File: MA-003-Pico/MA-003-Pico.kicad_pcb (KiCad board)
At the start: 2 copper layers, 49.5 x 80 mm, 5 parts, among them M1 rs485_ttl_module, M2 rs485_ttl_module, M3 rs485_ttl_module, M4 rs485_ttl_module

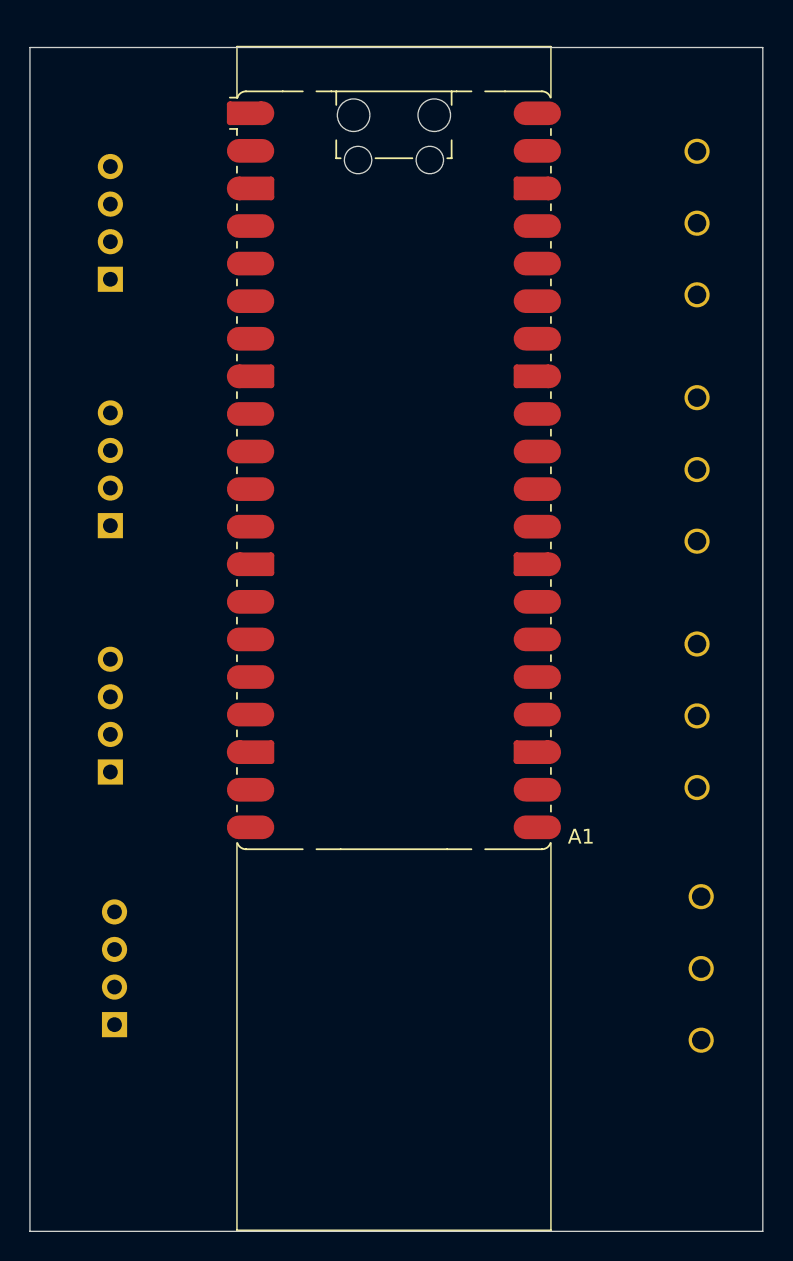
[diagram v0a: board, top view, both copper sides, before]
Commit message: Some more work
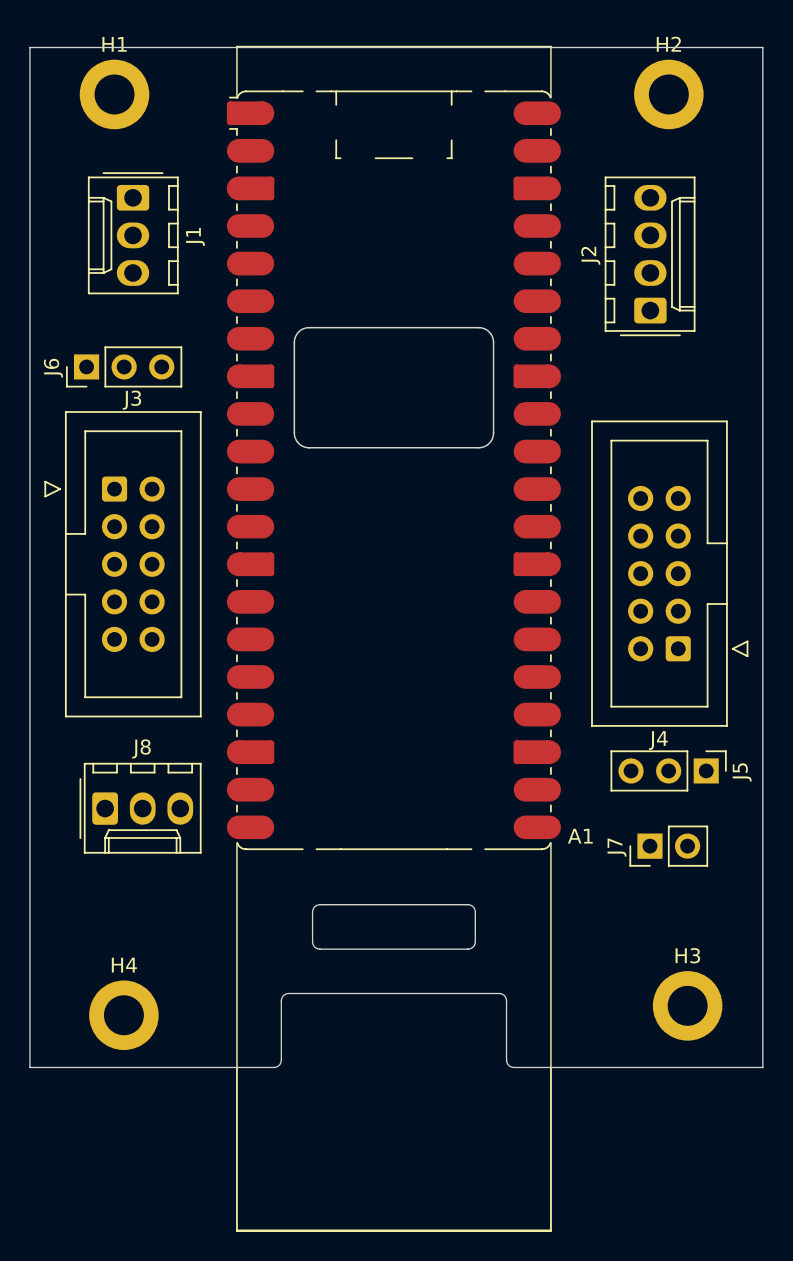
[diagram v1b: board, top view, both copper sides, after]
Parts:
- removed M1, M2, M3, M4: rs485_ttl_module, RS485ToTTL:rs485_ttl_module
- added H1: MountingHole_Pad, MountingHole:MountingHole_2.7mm_M2.5_DIN965_Pad, F.Cu at (138.4, 61.6)
- added H2: MountingHole_Pad, MountingHole:MountingHole_2.7mm_M2.5_DIN965_Pad, F.Cu at (175.9, 61.6)
- added H3: MountingHole_Pad, MountingHole:MountingHole_2.7mm_M2.5_DIN965_Pad, F.Cu at (177.2, 123.2)
- added H4: MountingHole_Pad, MountingHole:MountingHole_2.7mm_M2.5_DIN965_Pad, F.Cu at (139.1, 123.8)
- added J1: Power, Connector_Molex:Molex_KK-254_AE-6410-03A_1x03_P2.54mm_Vertical, F.Cu at (139.7, 68.6)
- added J2: I2C, Connector_Molex:Molex_KK-254_AE-6410-04A_1x04_P2.54mm_Vertical, F.Cu at (174.6, 76.2)
- added J3: Interface_A, Connector_IDC:IDC-Header_2x05_P2.54mm_Vertical, F.Cu at (138.4, 88.3)
- added J4: Interface_B, Connector_IDC:IDC-Header_2x05_P2.54mm_Vertical, F.Cu at (176.5, 99.1)
- added J5: Power_IB, Connector_PinHeader_2.54mm:PinHeader_1x03_P2.54mm_Vertical, F.Cu at (178.4, 107.3)
- added J6: Power_IA, Connector_PinHeader_2.54mm:PinHeader_1x03_P2.54mm_Vertical, F.Cu at (136.5, 80.0)
- added J7: Pico_On/Off, Connector_PinHeader_2.54mm:PinHeader_1x02_P2.54mm_Vertical, F.Cu at (174.6, 112.4)
- added J8: WS2812, Connector_Molex:Molex_KK-254_AE-6410-03A_1x03_P2.54mm_Vertical, F.Cu at (137.8, 109.9)
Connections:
- A1 pad 1: unconnected-(A1-GPIO0-Pad1) -> /GPIO_1
- A1 pad 10: unconnected-(A1-GPIO7-Pad10) -> /GPIO_8
- A1 pad 11: unconnected-(A1-GPIO8-Pad11) -> /GPIO_9
- A1 pad 12: unconnected-(A1-GPIO9-Pad12) -> /GPIO_10
- A1 pad 13: Net-(A1-GND-Pad13) -> /GND
- A1 pad 14: unconnected-(A1-GPIO10-Pad14) -> /GPIO_11
- A1 pad 15: unconnected-(A1-GPIO11-Pad15) -> /GPIO_12
- A1 pad 16: unconnected-(A1-GPIO12-Pad16) -> /GPIO_13
- A1 pad 17: unconnected-(A1-GPIO13-Pad17) -> /GPIO_14
- A1 pad 18: Net-(A1-GND-Pad13) -> /GND
- A1 pad 19: unconnected-(A1-GPIO14-Pad19) -> /GPIO_15
- A1 pad 2: unconnected-(A1-GPIO1-Pad2) -> /GPIO_2
- A1 pad 20: unconnected-(A1-GPIO15-Pad20) -> /GPIO_16
- A1 pad 23: Net-(A1-GND-Pad13) -> /GND
- A1 pad 28: Net-(A1-GND-Pad13) -> /GND
- A1 pad 3: Net-(A1-GND-Pad13) -> /GND
- A1 pad 30: unconnected-(A1-RUN-Pad30) -> Net-(A1-RUN)
- A1 pad 31: unconnected-(A1-GPIO26_ADC0-Pad31) -> /I2C_SDA
- A1 pad 32: unconnected-(A1-GPIO27_ADC1-Pad32) -> /I2C_SCL
- A1 pad 33: unconnected-(A1-AGND-Pad33) -> /GND
- A1 pad 34: unconnected-(A1-GPIO28_ADC2-Pad34) -> Net-(A1-GPIO28_ADC2)
- A1 pad 38: Net-(A1-GND-Pad13) -> /GND
- A1 pad 39: unconnected-(A1-VSYS-Pad39) -> /5V
- A1 pad 4: unconnected-(A1-GPIO2-Pad4) -> /GPIO_3
- A1 pad 5: unconnected-(A1-GPIO3-Pad5) -> /GPIO_4
- A1 pad 6: unconnected-(A1-GPIO4-Pad6) -> /GPIO_5
- A1 pad 7: unconnected-(A1-GPIO5-Pad7) -> /GPIO_6
- A1 pad 8: Net-(A1-GND-Pad13) -> /GND
- A1 pad 9: unconnected-(A1-GPIO6-Pad9) -> /GPIO_7
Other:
- board size 49.5 x 80 mm -> 49.5 x 68.9 mm

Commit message: Finishing the dmx ethernet pico
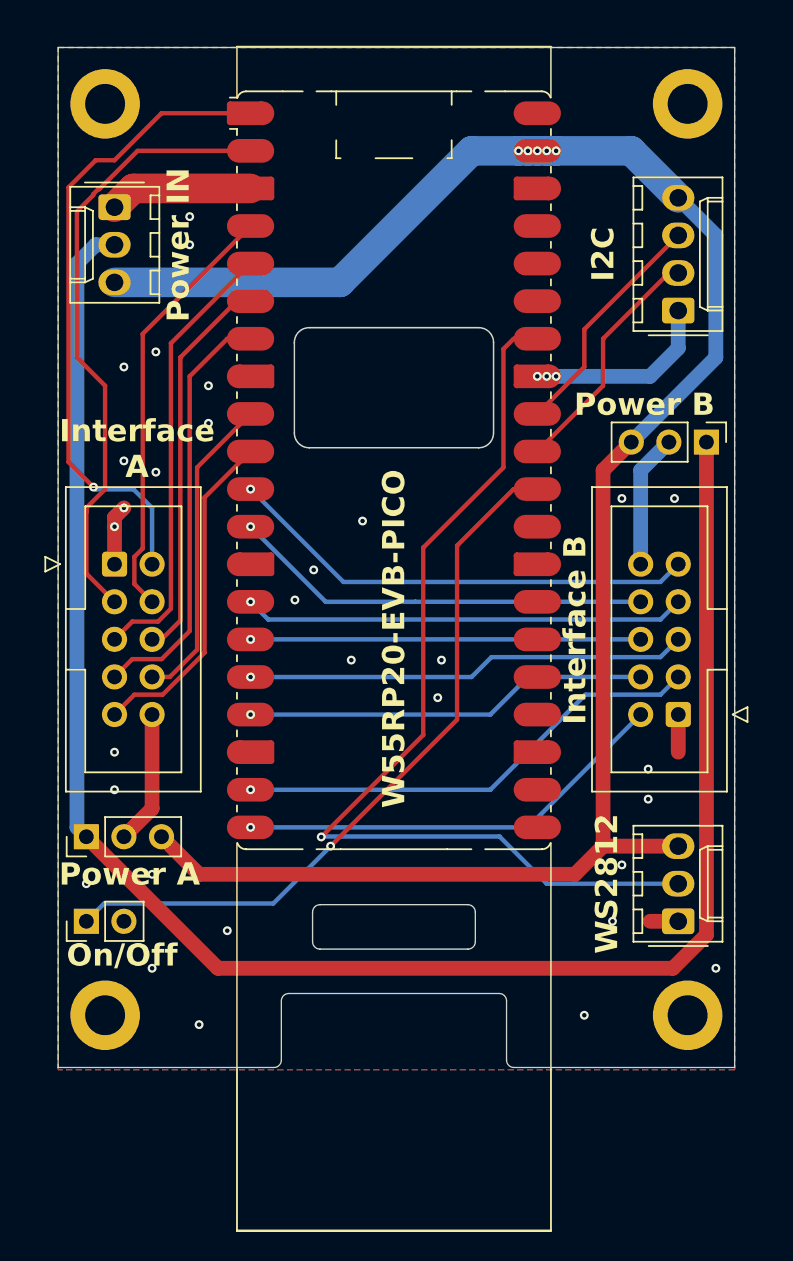
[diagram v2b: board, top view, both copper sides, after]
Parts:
- J1: value Power -> Power IN
- J3: value Interface_A -> Interface A
- moved J8 39.5 mm to (176.5, 117.5), turned to 90 degrees
- moved J7 38.4 mm to (136.5, 117.5)
- moved J6 31.8 mm to (136.5, 111.8)
- moved J5 22.2 mm to (178.4, 85.1)
- moved J3 5.08 mm to (138.4, 93.3)
- moved J4 4.44 mm to (176.5, 103.5)
- moved J2 1.88 mm to (176.5, 76.2)
- moved H2 1.42 mm to (177.2, 62.2)
- moved J1 1.40 mm to (138.4, 69.2)
- moved H4 1.27 mm to (137.8, 123.8)
- moved H1 0.90 mm to (137.8, 62.2)
- moved H3 0.64 mm to (177.2, 123.8)
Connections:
- J4 pad 2: /GPIO_9 -> /GPIO_16
- J4 pad 3: /GPIO_10 -> /GPIO_15
- J4 pad 4: /GPIO_11 -> /GPIO_14
- J4 pad 5: /GPIO_12 -> /GPIO_13
- J4 pad 6: /GPIO_13 -> /GPIO_12
- J4 pad 7: /GPIO_14 -> /GPIO_11
- J4 pad 8: /GPIO_15 -> /GPIO_10
- J4 pad 9: /GPIO_16 -> /GPIO_9
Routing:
- net /5V: track 0.00 -> 127.9 mm, vias 0 -> 5
- net /3V3: track 0.00 -> 121.9 mm
- net Net-(A1-GPIO28_ADC2): track 0.00 -> 66.1 mm, vias 0 -> 1
- net Net-(A1-RUN): track 0.00 -> 49.5 mm, vias 0 -> 1
- net /GPIO_1: track 0.00 -> 43.7 mm, vias 0 -> 1
- net /GPIO_2: track 0.00 -> 42.0 mm
- net /GPIO_15: track 0.00 -> 32.1 mm, vias 0 -> 1
- net /GPIO_9: track 0.00 -> 32.0 mm, vias 0 -> 1
- net /GND: track 0.00 -> 31.1 mm, vias 0 -> 34
- net /GPIO_4: track 0.00 -> 30.2 mm
- net /GPIO_13: track 0.00 -> 30.0 mm, vias 0 -> 1
- net /GPIO_11: track 0.00 -> 29.9 mm, vias 0 -> 1
- net /GPIO_16: track 0.00 -> 29.5 mm, vias 0 -> 1
- net /GPIO_3: track 0.00 -> 29.1 mm
- net /GPIO_6: track 0.00 -> 28.7 mm
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- added copper zone on B.Cu, net /GND
- added copper zone on F.Cu, net /GND
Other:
- board size 49.5 x 68.9 mm -> 45.7 x 68.9 mm
- board text added: "I2C"
- board text added: "Interface A"
- board text added: "Interface B"
- board text added: "On/Off"
- board text added: "Power A"
- board text added: "Power B"
- board text added: "W55RP20-EVB-PICO"
- board text added: "WS2812"
